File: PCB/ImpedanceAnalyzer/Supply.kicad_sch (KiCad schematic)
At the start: 0 parts

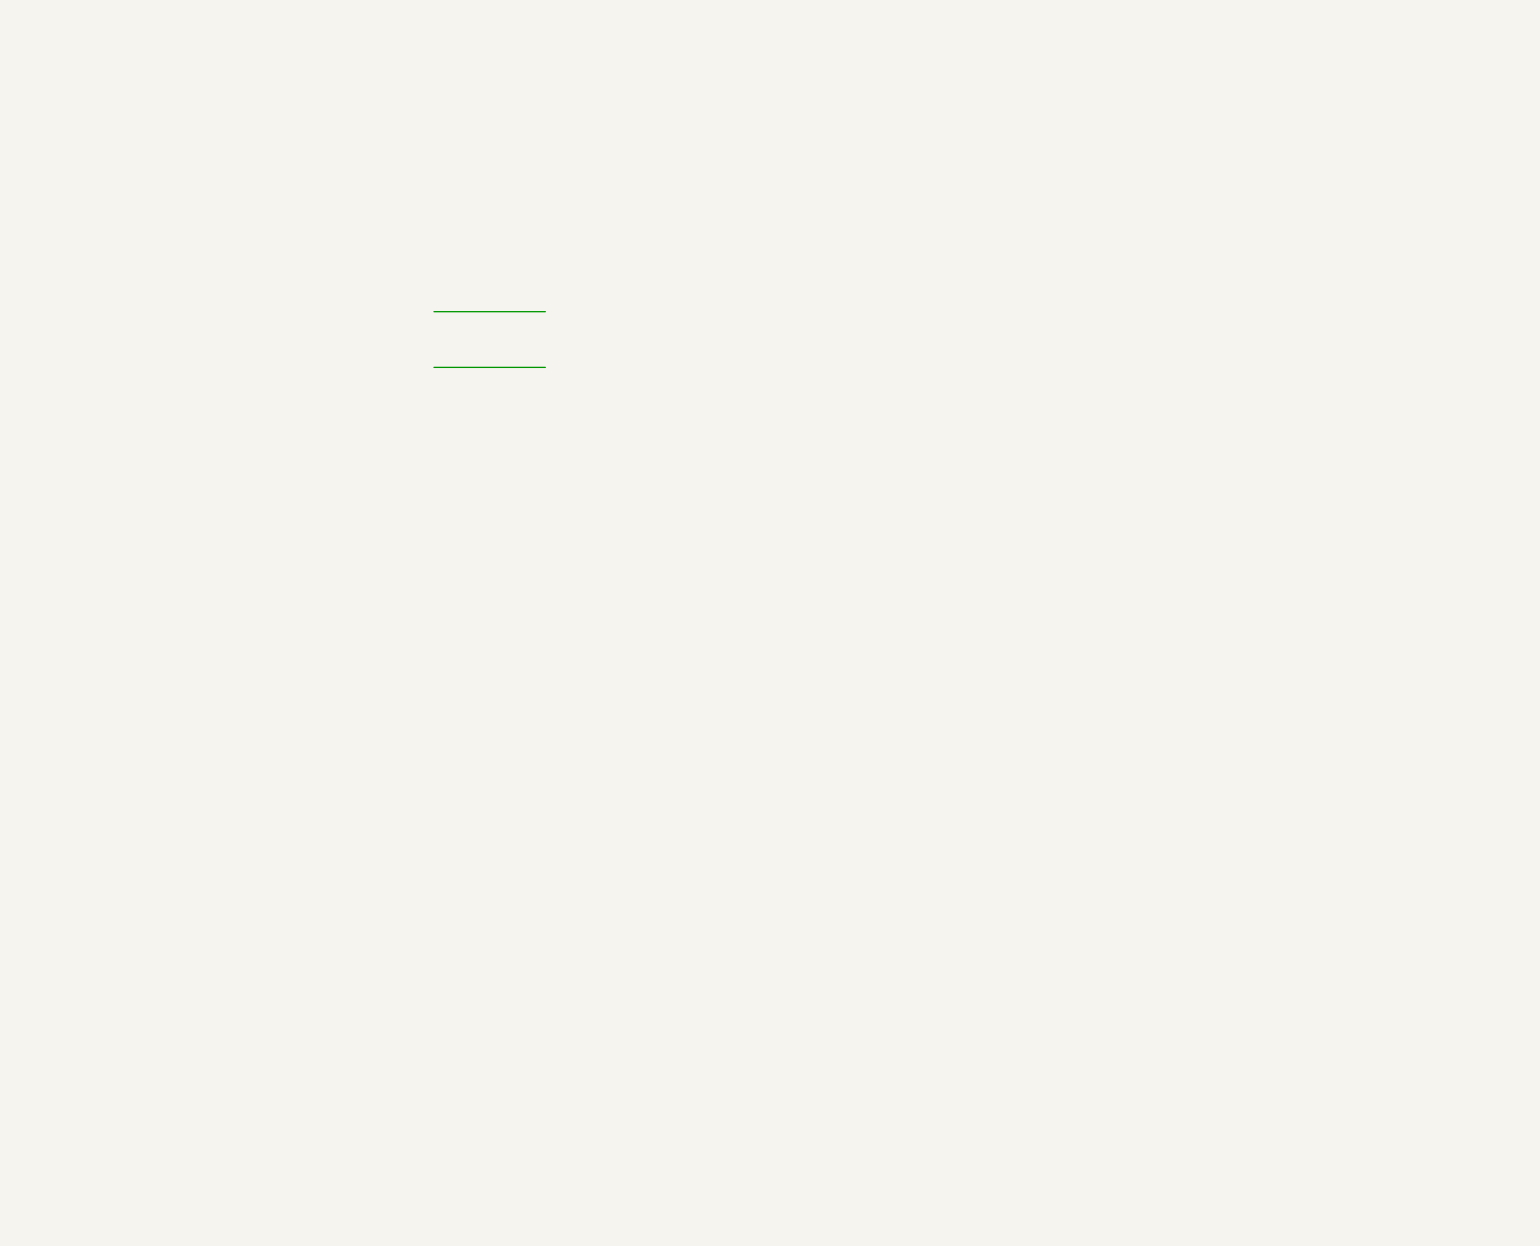
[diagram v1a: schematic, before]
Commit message: schematic v1
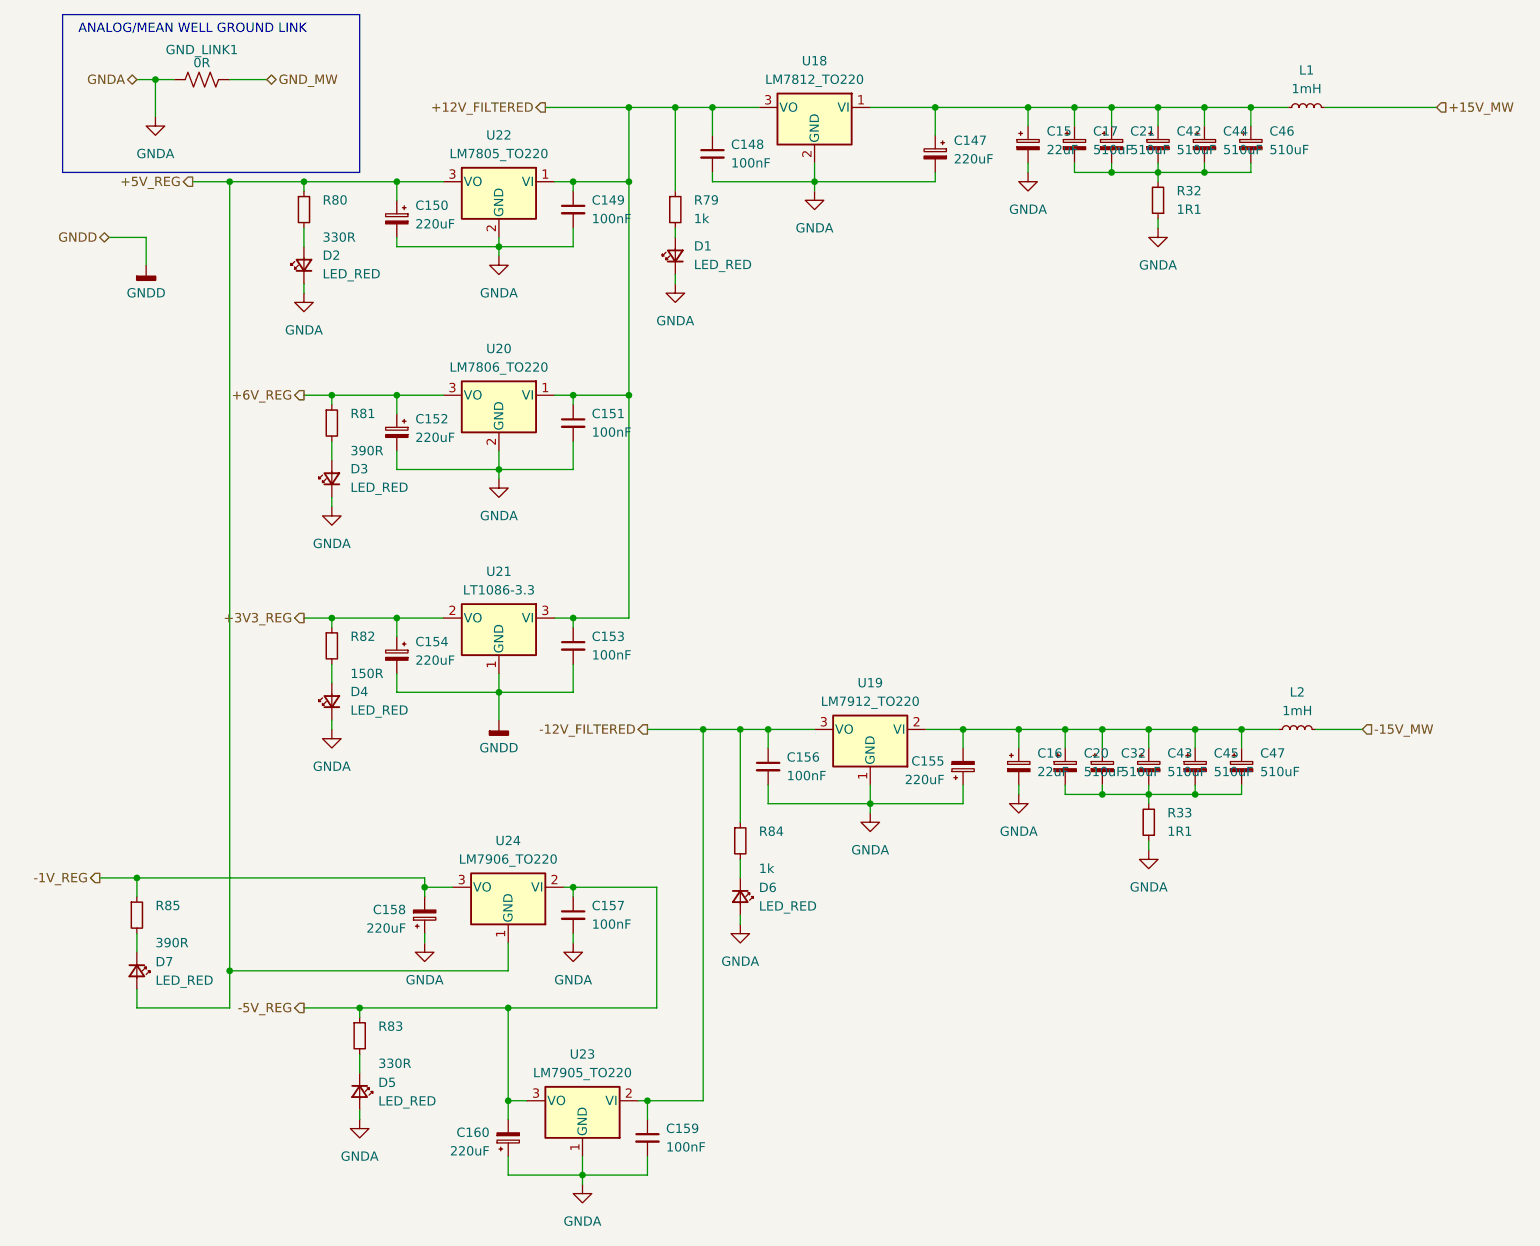
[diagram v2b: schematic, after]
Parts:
- added C147, C150, C152, C154, C155, C158, C160: 220uF, symbol Device:C_Polarized_Small
- added C148, C149, C151, C153, C156, C157, C159: 100nF, symbol Device:C_Small
- added C15, C16: 22uF, symbol Device:C_Polarized_Small
- added C17, C20, C21, C32, C42, C43, C44, C45, C46, C47: 510uF, symbol Device:C_Polarized_Small
- added D1, D2, D3, D4, D5, D6, D7: LED_RED, symbol Device:LED_Small
- added GND_LINK1: 0R, symbol Device:R_US
- added L1, L2: 1mH, symbol Device:L_Small
- added R32, R33: 1R1, symbol Device:R_Small
- added R79, R84: 1k, symbol Device:R_Small
- added R80, R83: 330R, symbol Device:R_Small
- added R81, R85: 390R, symbol Device:R_Small
- added R82: 150R, symbol Device:R_Small
- added U18: LM7812_TO220, Package_TO_SOT_THT:TO-220-3_Vertical, symbol Regulator_Linear:LM7812_TO220
- added U19: LM7912_TO220, Package_TO_SOT_THT:TO-220-3_Vertical, symbol Regulator_Linear:LM7912_TO220
- added U20: LM7806_TO220, Package_TO_SOT_THT:TO-220-3_Vertical, symbol Regulator_Linear:LM7806_TO220
- added U21: LT1086-3.3, symbol Regulator_Linear:LT1086-3.3
- added U22: LM7805_TO220, Package_TO_SOT_THT:TO-220-3_Vertical, symbol Regulator_Linear:LM7805_TO220
- added U23: LM7905_TO220, Package_TO_SOT_THT:TO-220-3_Vertical, symbol Regulator_Linear:LM7905_TO220
- added U24: LM7906_TO220, Package_TO_SOT_THT:TO-220-3_Vertical, symbol Regulator_Linear:LM7906_TO220
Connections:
- new net: D1.2 (A), R79.2
- new net: D6.1 (K), R84.2
- new net: D2.2 (A), R80.2
- new net: D4.2 (A), R82.2
- new net: D5.1 (K), R83.2
- new net: C147.1, C15.1, C17.1, C21.1, C42.1, C44.1, C46.1, L1.1, U18.1 (VI)
- new net: C17.2, C21.2, C42.2, C44.2, C46.2, R32.2
- new net: C155.2, C16.1, C20.1, C32.1, C43.1, C45.1, C47.1, L2.1, U19.2 (VI)
- new net: C20.2, C32.2, C43.2, C45.2, C47.2, R33.2
- new net: D7.1 (K), R85.2
- new net: D3.2 (A), R81.2
- new net +12V_FILTERED: C148.1, C149.1, C151.1, C153.1, R79.1, U18.3 (VO), U20.1 (VI), U21.3 (VI), U22.1 (VI)
- new net +15V_MW: L1.2
- new net +3V3_REG: C154.1, R82.1, U21.2 (VO)
- new net +5V_REG: C150.1, D7.2 (A), R80.1, U22.3 (VO), U24.1 (GND)
- new net +6V_REG: C152.1, R81.1, U20.3 (VO)
- new net -12V_FILTERED: C156.1, C159.1, R84.1, U19.3 (VO), U23.2 (VI)
- new net -15V_MW: L2.2
- new net -1V_REG: C158.2, R85.1, U24.3 (VO)
- new net -5V_REG: C157.1, C160.2, R83.1, U23.3 (VO), U24.2 (VI)
- new net GNDA: C147.2, C148.2, C149.2, C15.2, C150.2, C151.2, C152.2, C155.1, C156.2, C157.2, C158.1, C159.2, C16.2, C160.1, D1.1 (K), D2.1 (K), D3.1 (K), D4.1 (K), D5.2 (A), D6.2 (A), GND_LINK1.1, R32.1, R33.1, U18.2 (GND), U19.1 (GND), U20.2 (GND), U22.2 (GND), U23.1 (GND)
- new net GNDD: C153.2, C154.2, U21.1 (GND)
- new net GND_MW: GND_LINK1.2
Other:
- note added: "ANALOG/MEAN WELL GROUND LINK"
